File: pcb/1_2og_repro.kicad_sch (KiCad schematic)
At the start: 29 parts, among them J1 Pico EzMate, J2 548190519, J3 RAW, J4 S3B, Q1 2N7002, SW95 SW_Push, U1 XC6206PxxxMR, U2 STM32F072C8Tx, U3 SRV05-4, U4 74AHCT1G125

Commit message: update gerbers, change mounting hole dimensions
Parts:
- H1, H2: footprint MountingHole:MountingHole_3.2mm_M3_Pad -> MountingHole:MountingHole_3mm_Pad
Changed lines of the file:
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@@
       (effects (font (size 1.27 1.27)) (justify left) hide)
     )
-    (property "Footprint" "MountingHole:MountingHole_3.2mm_M3_Pad" (at 165.227 19.304 0)
+    (property "Footprint" "MountingHole:MountingHole_3mm_Pad" (at 165.227 19.304 0)
       (effects (font (size 1.27 1.27)) hide)
     )
@@
       (effects (font (size 1.27 1.27)) (justify right) hide)
     )
-    (property "Footprint" "MountingHole:MountingHole_3.2mm_M3_Pad" (at 170.307 19.304 0)
+    (property "Footprint" "MountingHole:MountingHole_3mm_Pad" (at 170.307 19.304 0)
       (effects (font (size 1.27 1.27)) hide)
     )

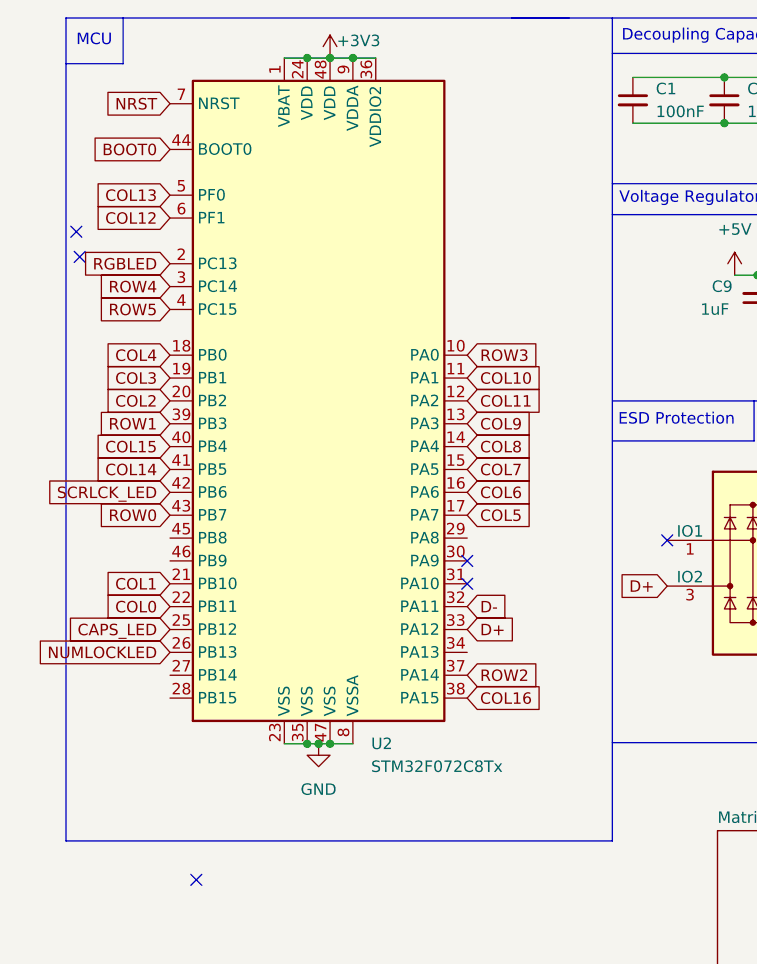
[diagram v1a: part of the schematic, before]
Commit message: ok juggle a few pins around
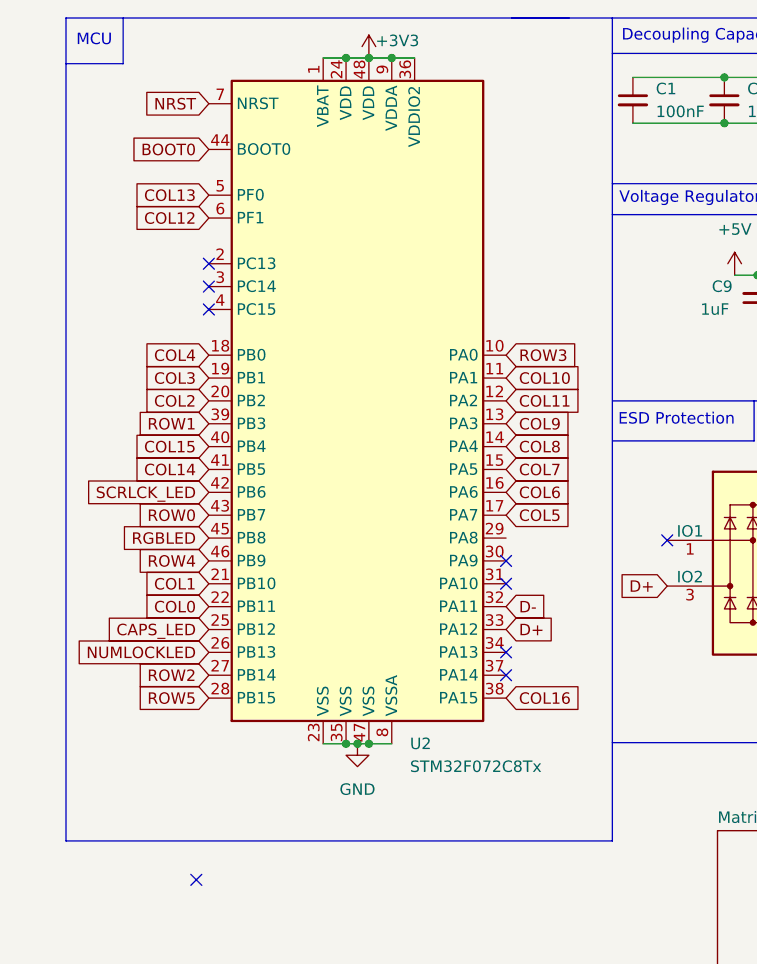
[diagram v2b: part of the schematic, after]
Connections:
- net RGBLED: now also U2.45 (PB8); no longer U2.2 (PC13)
- net ROW2: now also U2.27 (PB14); no longer U2.37 (PA14)
- net ROW4: now also U2.46 (PB9); no longer U2.3 (PC14)
- net ROW5: now also U2.28 (PB15); no longer U2.4 (PC15)
- no-connect marks 8 -> 11
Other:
- moved on the sheet: U2
